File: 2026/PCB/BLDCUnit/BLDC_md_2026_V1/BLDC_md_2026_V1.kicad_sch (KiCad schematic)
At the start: 67 parts, among them J1 Conn_01x07_Pin, J2 Conn_01x02_Pin, J3 Conn_01x03_Socket, J4 Conn_01x02_Socket, SW1 SW_MEC_5E, SW2 SW_MEC_5E, U1 MAX3051

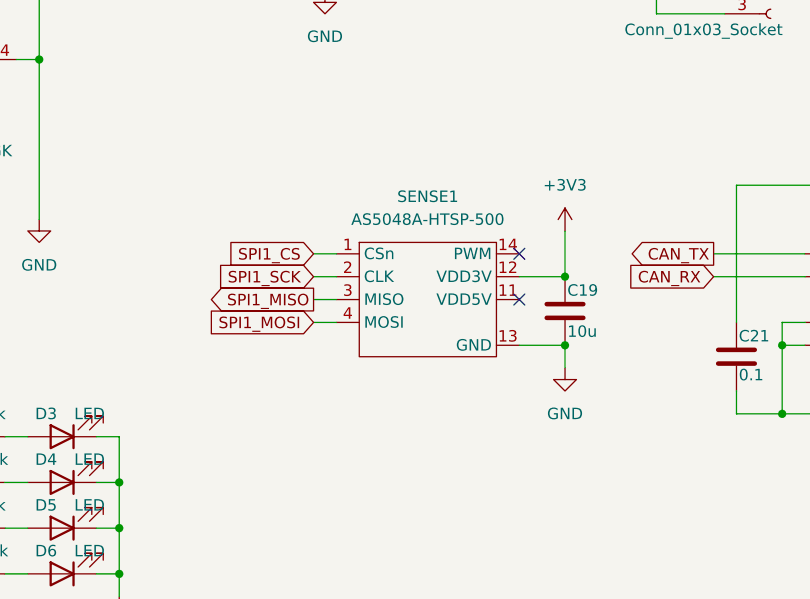
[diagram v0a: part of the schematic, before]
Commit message: PCBレイアウト開始
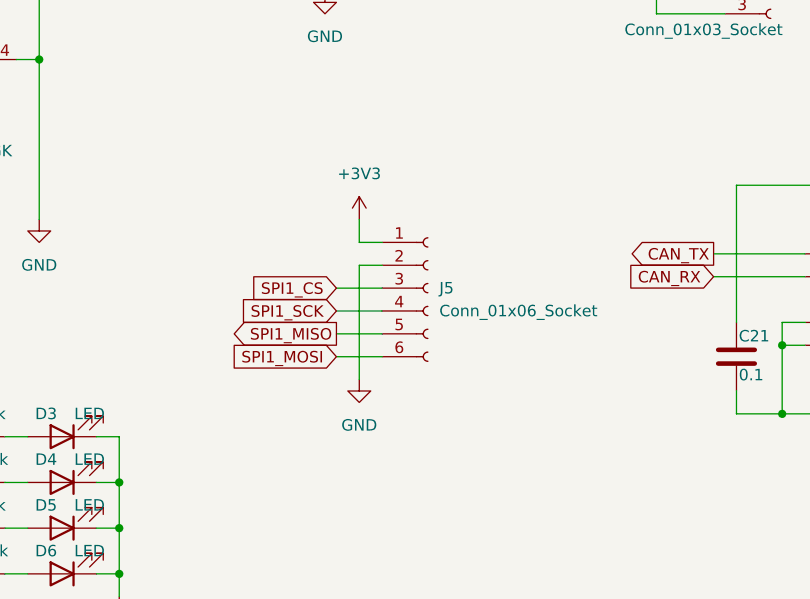
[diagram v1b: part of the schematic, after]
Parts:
- removed C19: 10u, Capacitor_SMD:C_1210_3225Metric_Pad1.33x2.70mm_HandSolder, symbol Device:C
- removed SENSE1: AS5048A-HTSP-500, Package_SO:TSSOP-14_4.4x5mm_P0.65mm, symbol BLDCUnit_LIB_SYM:AS5048A-HTSP-500
- added J5: Conn_01x06_Socket, Connector_JST:JST_PH_S6B-PH-K_1x06_P2.00mm_Horizontal, symbol Connector:Conn_01x06_Socket
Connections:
- net +3V3: now also J5.1 (Pin_1)
- net GND: now also J5.2 (Pin_2)
- net SPI1_CS: now also J5.3 (Pin_3)
- net SPI1_MISO: now also J5.5 (Pin_5)
- net SPI1_MOSI: now also J5.6 (Pin_6)
- net SPI1_SCK: now also J5.4 (Pin_4)
- no-connect marks 2 -> 0

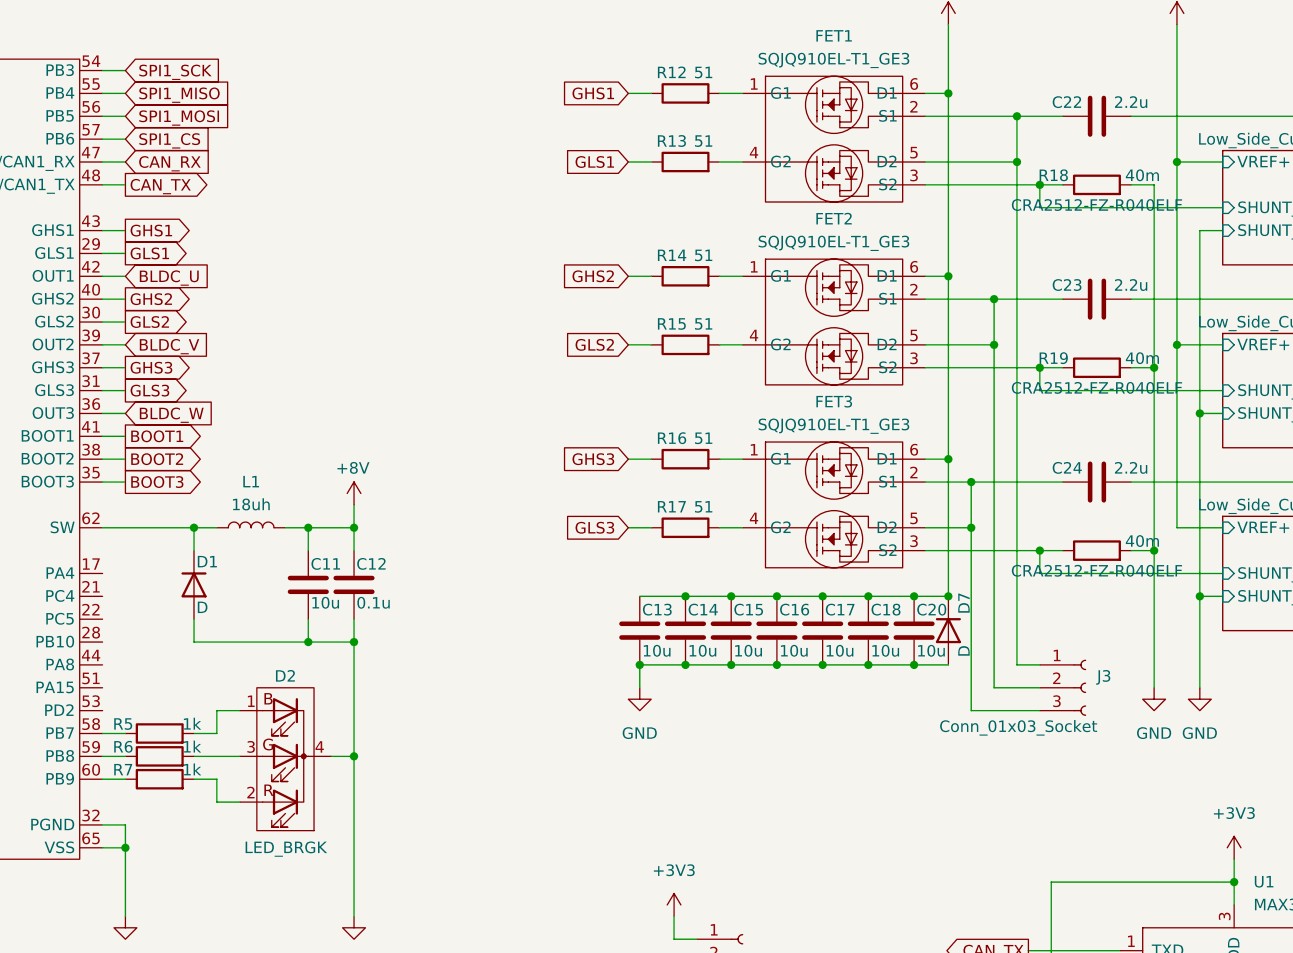
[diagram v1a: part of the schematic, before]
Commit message: U,V,W生やした
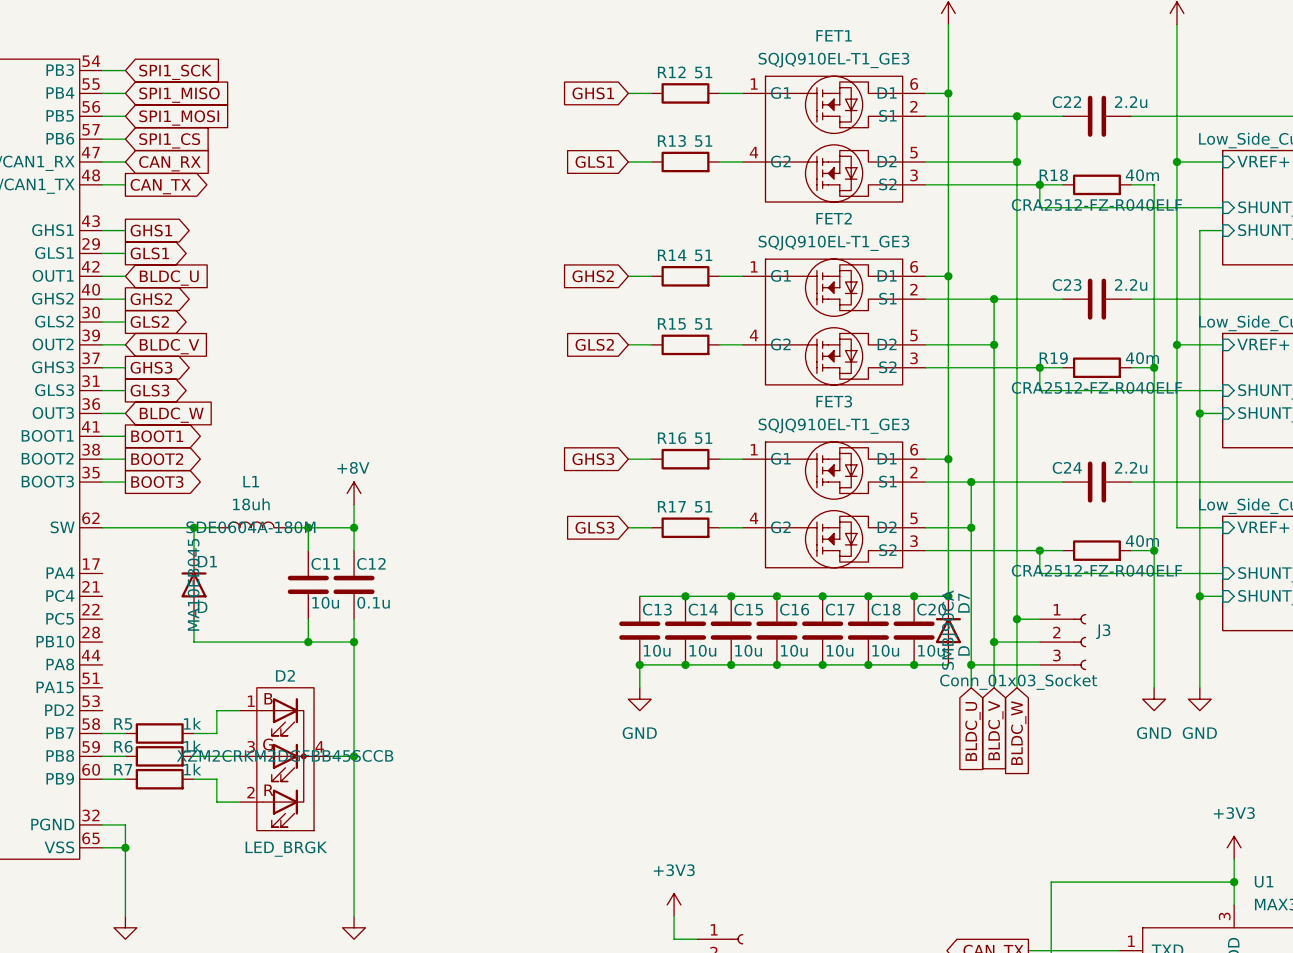
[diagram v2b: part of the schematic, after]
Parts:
- D1: footprint Diode_SMD:D_SMB -> BLDCUint_LIB_FTP:MA10EB045
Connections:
- net BLDC_U: now also C24.1, FET3.2 (S1), FET3.5 (D2), J3.3 (Pin_3)
- net BLDC_V: now also C23.1, FET2.2 (S1), FET2.5 (D2), J3.2 (Pin_2)
- net BLDC_W: now also C22.1, FET1.2 (S1), FET1.5 (D2), J3.1 (Pin_1)
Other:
- moved on the sheet: J3
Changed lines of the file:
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@@
 	)
 	(junction
-		(at 203.2 59.69)
-		(diameter 0)
-		(color 0 0 0 0)
-	)
-	(junction
 		(at 50.8 80.01)
 		(diameter 0)
@@
 	)
 	(junction
-		(at 43.18 41.91)
+		(at 205.74 90.17)
 		(diameter 0)
 		(color 0 0 0 0)
 	)
 	(junction
-		(at 140.97 157.48)
+		(at 43.18 41.91)
 		(diameter 0)
 		(color 0 0 0 0)
 	)
 	(junction
-		(at 189.23 95.25)
+		(at 140.97 157.48)
 		(diameter 0)
 		(color 0 0 0 0)
 	)
 	(junction
-		(at 189.23 87.63)
+		(at 189.23 95.25)
 		(diameter 0)
 		(color 0 0 0 0)
 	)
 	(junction
-		(at 205.74 39.37)
+		(at 189.23 87.63)
 		(diameter 0)
 		(color 0 0 0 0)
@@
 	)
 	(junction
+		(at 200.66 80.01)
+		(diameter 0)
+		(color 0 0 0 0)
+	)
+	(junction
 		(at 205.74 34.29)
 		(diameter 0)
@@
 	)
 	(junction
+		(at 200.66 95.25)
+		(diameter 0)
+		(color 0 0 0 0)
+	)
+	(junction
 		(at 184.15 87.63)
 		(diameter 0)
@@
 	)
 	(junction
+		(at 203.2 92.71)
+		(diameter 0)
+		(color 0 0 0 0)
+	)
+	(junction
 		(at 40.64 85.09)
 		(diameter 0)
@@
 	)
 	(junction
-		(at 200.66 80.01)
-		(diameter 0)
-		(color 0 0 0 0)
-	)
-	(junction
 		(at 229.87 144.78)
 		(diameter 0)
@@
 	)
 	(junction
+		(at 203.2 59.69)
+		(diameter 0)
+		(color 0 0 0 0)
+	)
+	(junction
 		(at 52.07 166.37)
 		(diameter 0)
@@
 	)
 	(junction
+		(at 205.74 39.37)
+		(diameter 0)
+		(color 0 0 0 0)
+	)
+	(junction
 		(at 63.5 24.13)
 		(diameter 0)
@@
 	(wire
 		(pts
-			(xy 200.66 100.33) (xy 208.28 100.33)
+			(xy 200.66 95.25) (xy 208.28 95.25)
 		)
 		(stroke
@@
 	(wire
 		(pts
+			(xy 200.66 80.01) (xy 200.66 95.25)
+		)
+		(stroke
+			(width 0)
+			(type default)
+		)
+	)
+	(wire
+		(pts
 			(xy 104.14 59.69) (xy 106.68 59.69)
 		)
@@
 	(wire
 		(pts
-			(xy 200.66 80.01) (xy 200.66 100.33)
-		)
-		(stroke
-			(width 0)
-			(type default)
-		)
-	)
-	(wire
-		(pts
 			(xy 198.12 31.75) (xy 198.12 52.07)
 		)
@@
 	(wire
 		(pts
-			(xy 203.2 97.79) (xy 208.28 97.79)
+			(xy 203.2 92.71) (xy 208.28 92.71)
 		)
 		(stroke
@@
 	(wire
 		(pts
+			(xy 203.2 92.71) (xy 203.2 97.79)
+		)
+		(stroke
+			(width 0)
+			(type default)
+		)
+	)
+	(wire
+		(pts
 			(xy 63.5 29.21) (xy 63.5 31.75)
 		)
@@
 	(wire
 		(pts
+			(xy 205.74 39.37) (xy 205.74 90.17)
+		)
+		(stroke
+			(width 0)
+			(type default)
+		)
+	)
+	(wire
+		(pts
 			(xy 106.68 113.03) (xy 106.68 115.57)
 		)
@@
 	(wire
 		(pts
-			(xy 205.74 39.37) (xy 205.74 95.25)
-		)
-		(stroke
-			(width 0)
-			(type default)
-		)
-	)
-	(wire
-		(pts
 			(xy 33.02 41.91) (xy 38.1 41.91)
 		)
@@
 	(wire
 		(pts
-			(xy 205.74 95.25) (xy 208.28 95.25)
+			(xy 205.74 90.17) (xy 208.28 90.17)
 		)
 		(stroke
@@
 	(wire
 		(pts
+			(xy 200.66 95.25) (xy 200.66 97.79)
+		)
+		(stroke
+			(width 0)
+			(type default)
+		)
+	)
+	(wire
+		(pts
 			(xy 255.27 133.35) (xy 252.73 133.35)
 		)
@@
 	(wire
 		(pts
+			(xy 205.74 90.17) (xy 205.74 97.79)
+		)
+		(stroke
+			(width 0)
+			(type default)
+		)
+	)
+	(wire
+		(pts
 			(xy 140.97 147.32) (xy 140.97 152.4)
 		)
@@
 	(wire
 		(pts
-			(xy 203.2 59.69) (xy 203.2 97.79)
-		)
-		(stroke
-			(width 0)
-			(type default)
-		)
-	)
-	(wire
-		(pts
 			(xy 198.12 52.07) (xy 198.12 72.39)
 		)
@@
 	(wire
 		(pts
+			(xy 203.2 59.69) (xy 203.2 92.71)
+		)
+		(stroke
+			(width 0)
+			(type default)
+		)
+	)
+	(wire
+		(pts
 			(xy 104.14 115.57) (xy 106.68 115.57)
 		)
@@
 		)
 	)
+	(global_label "BLDC_U"
+		(shape input)
+		(at 200.66 97.79 270)
+		(fields_autoplaced yes)
+		(effects
+			(font
+				(size 1.27 1.27)
+			)
+			(justify right)
+		)
+		(property "Intersheetrefs" "${INTERSHEET_REFS}"
+			(at 200.66 107.9114 90)
+			(effects
+				(font
+					(size 1.27 1.27)
+				)
+				(justify right)
+				(hide yes)
+			)
+		)
+	)
 	(global_label "OP1_VINM"
 		(shape input)
@@
 		)
 	)
+	(global_label "BLDC_W"
+		(shape input)
+		(at 205.74 97.79 270)
+		(fields_autoplaced yes)
+		(effects
+			(font
+				(size 1.27 1.27)
+			)
+			(justify right)
+		)
+		(property "Intersheetrefs" "${INTERSHEET_REFS}"
+			(at 205.74 108.0323 90)
+			(effects
+				(font
+					(size 1.27 1.27)
+				)
+				(justify right)
+				(hide yes)
+			)
+		)
+	)
 	(global_label "USW"
 		(shape output)
@@
 		)
 	)
+	(global_label "BLDC_V"
+		(shape input)
+		(at 203.2 97.79 270)
+		(fields_autoplaced yes)
+		(effects
+			(font
+				(size 1.27 1.27)
+			)
+			(justify right)
+		)
+		(property "Intersheetrefs" "${INTERSHEET_REFS}"
+			(at 203.2 107.6695 90)
+			(effects
+				(font
+					(size 1.27 1.27)
+				)
+				(justify right)
+				(hide yes)
+			)
+		)
+	)
 	(global_label "USART_RX"
 		(shape input)
@@
 			)
 		)
-		(property "Footprint" "Diode_SMD:D_SMB"
+		(property "Footprint" "BLDCUint_LIB_FTP:MA10EB045"
 			(at 114.3 86.36 0)
 			(effects
@@
 			)
 		)
-		(property "Description" "Diode"
+		(property "Description" "MA10EB045"
 			(at 114.3 86.36 0)
 			(effects
@@
 					(size 1.27 1.27)
 				)
-				(hide yes)
 			)
 		)
@@
 		(on_board yes)
 		(dnp no)
-		(fields_autoplaced yes)
 		(property "Reference" "L1"
 			(at 120.65 74.93 90)
@@
 		)
 		(property "Description" "SDE0604A-180M"
-			(at 120.65 80.01 0)
+			(at 120.65 80.01 90)
 			(effects
 				(font
 					(size 1.27 1.27)
 				)
-				(hide yes)
 			)
 		)
@@
 	(symbol
 		(lib_id "Connector:Conn_01x03_Socket")
-		(at 213.36 97.79 0)
+		(at 213.36 92.71 0)
 		(unit 1)
 		(exclude_from_sim no)
@@
 		(dnp no)
 		(property "Reference" "J3"
-			(at 214.63 96.5199 0)
+			(at 214.63 91.4399 0)
 			(effects
 				(font
@@
 		)
 		(property "Value" "Conn_01x03_Socket"
-			(at 197.104 102.108 0)
+			(at 197.104 97.028 0)
 			(effects
 				(font
@@
 		)
 		(property "Footprint" "Connector_Molex:Molex_SPOX_5268-03A_1x03_P2.50mm_Horizontal"
-			(at 213.36 97.79 0)
+			(at 213.36 92.71 0)
 			(effects
 				(font
@@
 		)
 		(property "Datasheet" "~"
-			(at 213.36 97.79 0)
+			(at 213.36 92.71 0)
 			(effects
 				(font
@@
 		)
 		(property "Description" "Generic connector, single row, 01x03, script generated"
-			(at 213.36 97.79 0)
+			(at 213.36 92.71 0)
 			(effects
 				(font
@@
 					(size 1.27 1.27)
 				)
-				(hide yes)
 			)
 		)
@@
 			)
 		)
-		(property "Description" "Diode"
+		(property "Description" "SMBJ90CA"
 			(at 198.12 91.44 0)
 			(effects
@@
 					(size 1.27 1.27)
 				)
-				(hide yes)
 			)
 		)
